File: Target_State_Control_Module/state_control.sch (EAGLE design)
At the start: 30 parts, among them Q9 8MHz, U1 ATMEGA328P_PDIP, U2 FT232RLSSOP, X2 USBSMD

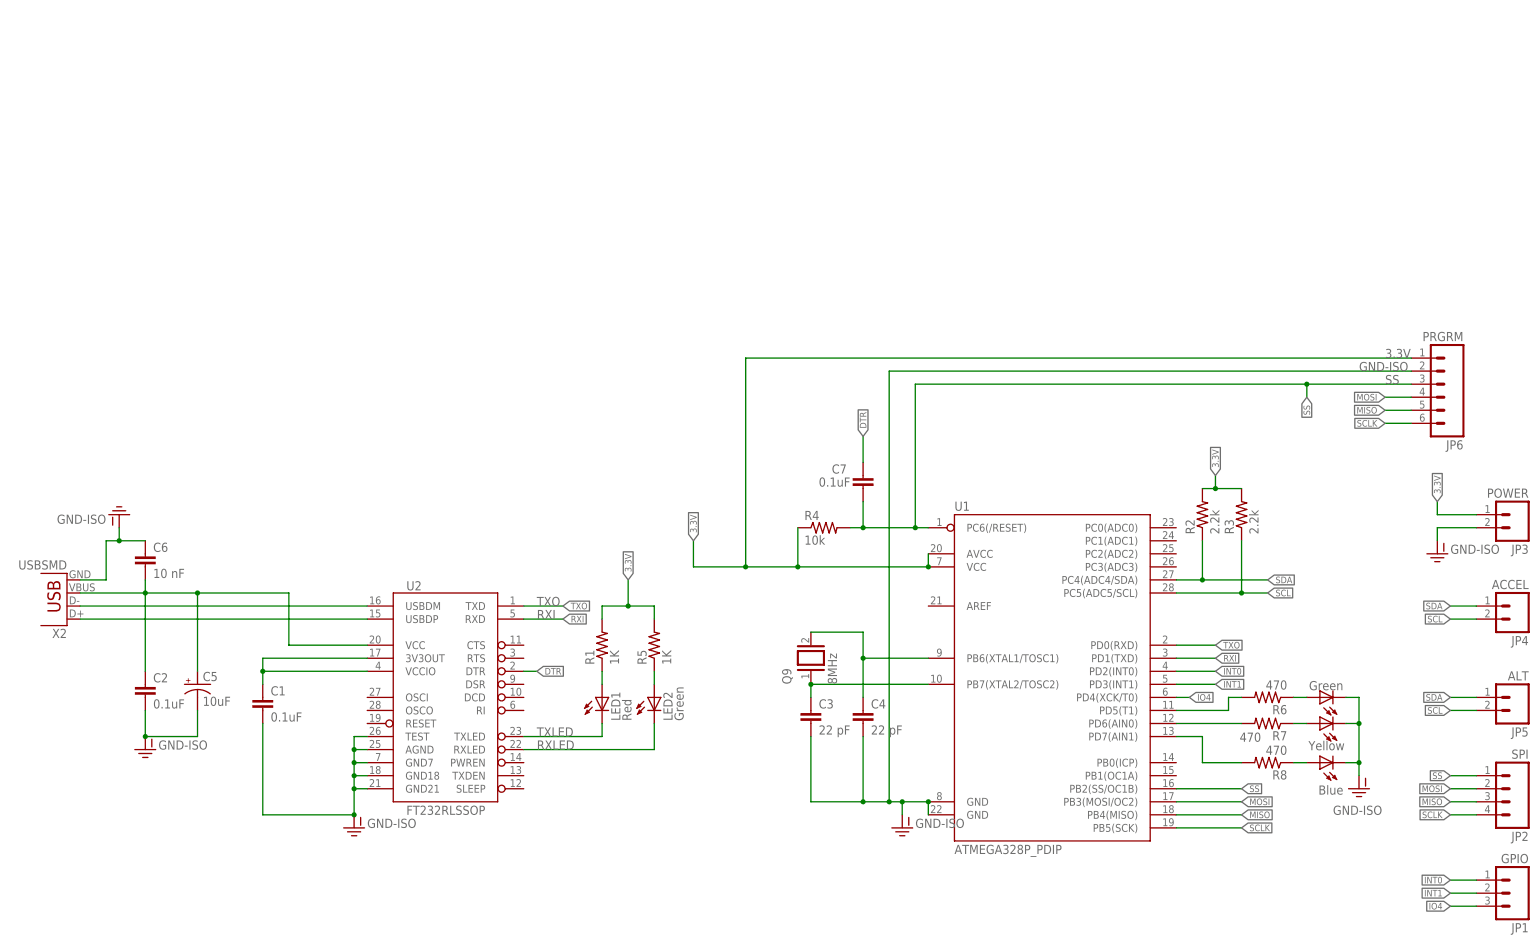
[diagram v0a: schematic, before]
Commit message: Some schematic updates
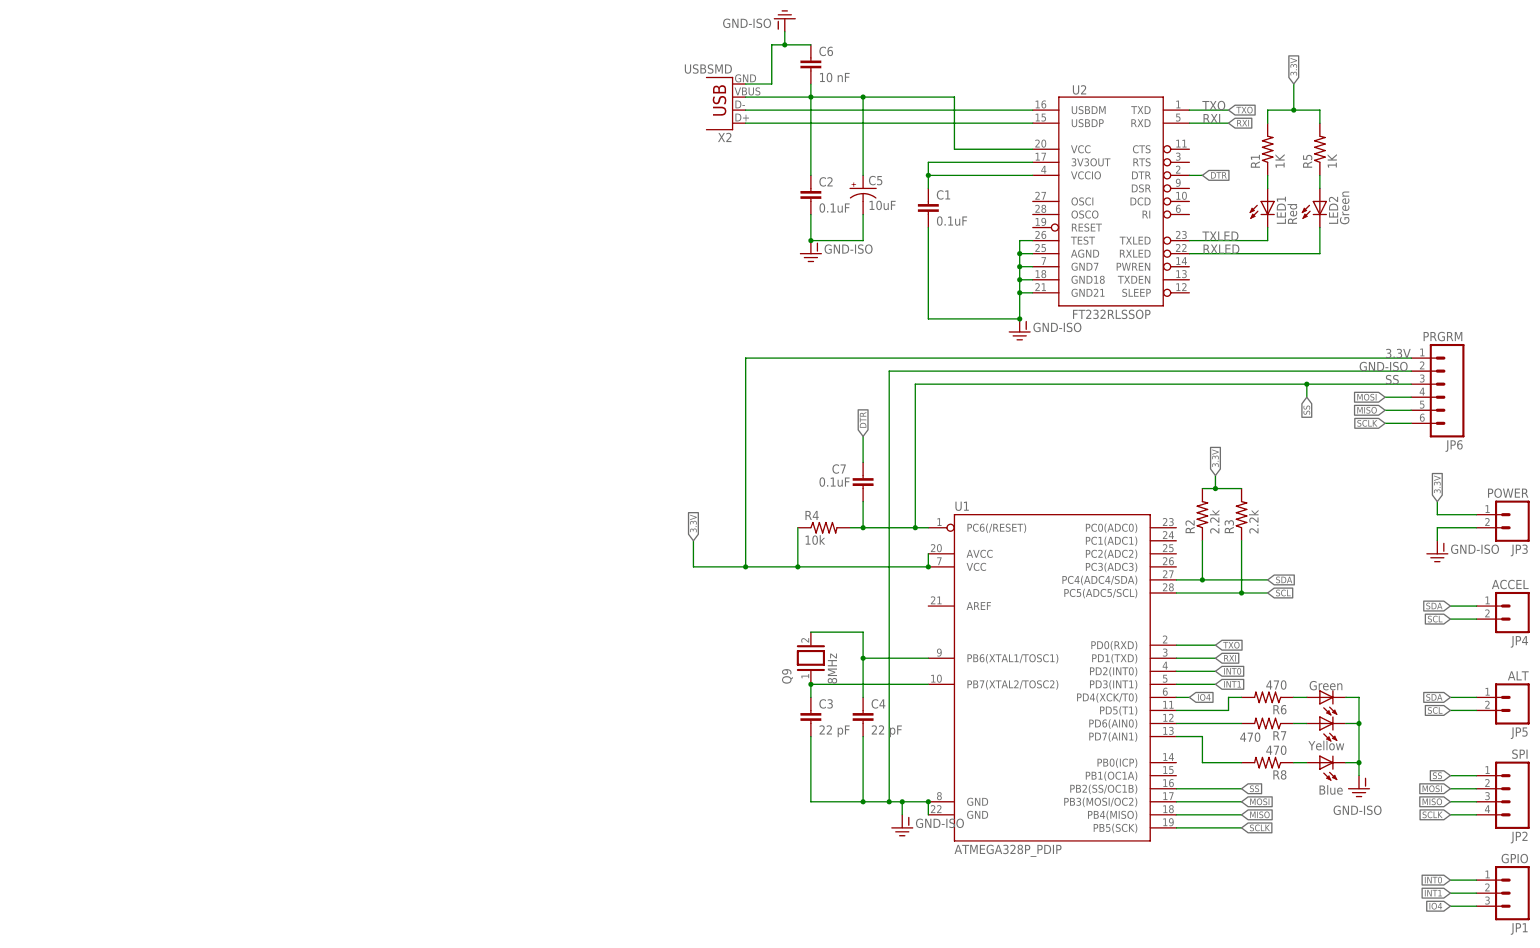
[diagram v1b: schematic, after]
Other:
- moved on the sheet: C1, C2, C5, C6, LED1, LED2, R1, R5, U2, X2
